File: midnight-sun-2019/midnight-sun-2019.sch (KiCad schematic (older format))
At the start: 71 parts, among them J1 Conn_02x02_Odd_Even, J2 USB_B_Micro, SW1 SW_SPDT, SW2 SW_SPDT, SW3 SW_SPDT, U1 74HC14, U10 74HC14, U11 74HC86, U12 74HC86, U13 74HC86, U14 74HC86, U15 74HC14, U16 74HC14, U2 74HC595, U3 74HC595, U4 74HC595, U5 74HC86, U6 74HC86, U7 74HC86, U8 74HC86, U9 74HC14

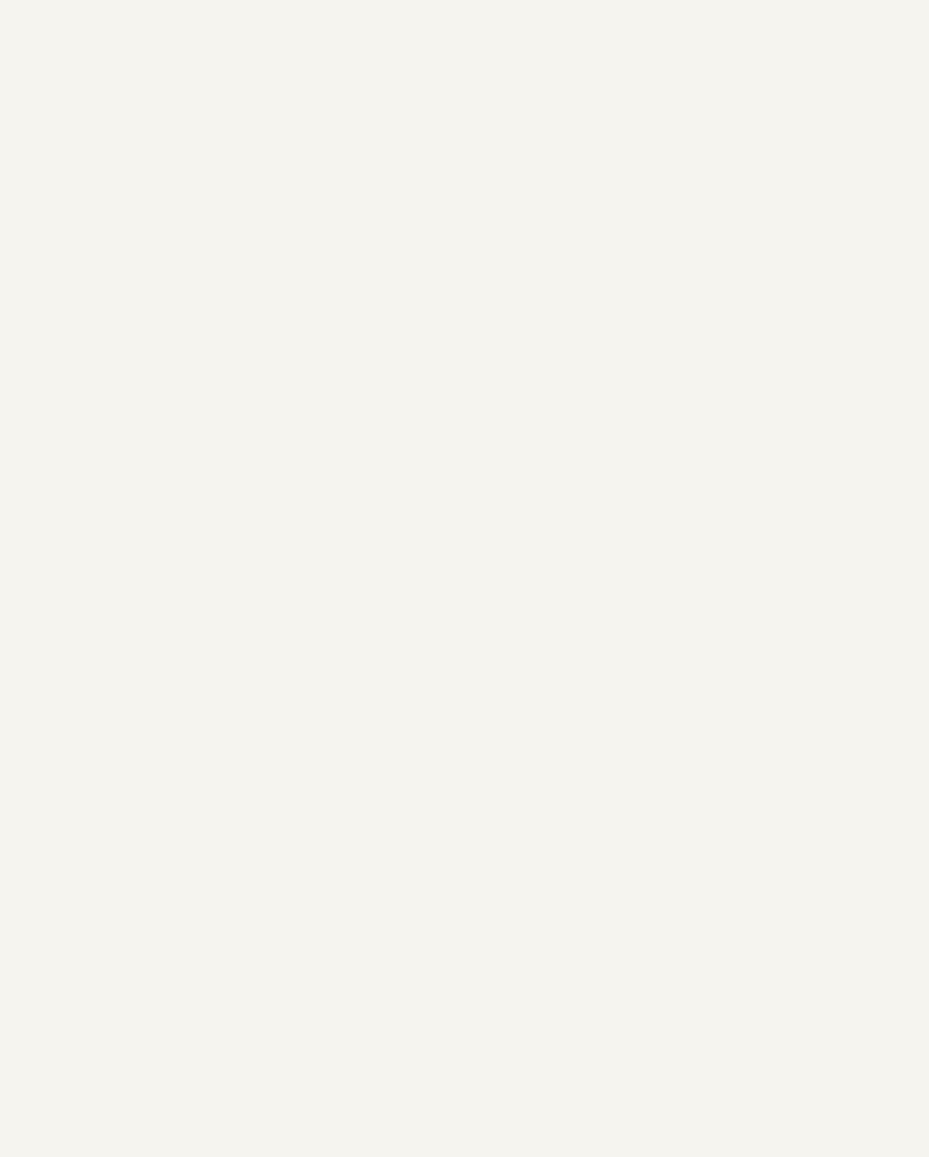
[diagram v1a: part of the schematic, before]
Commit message: Add GND and VCC connections to ICs...
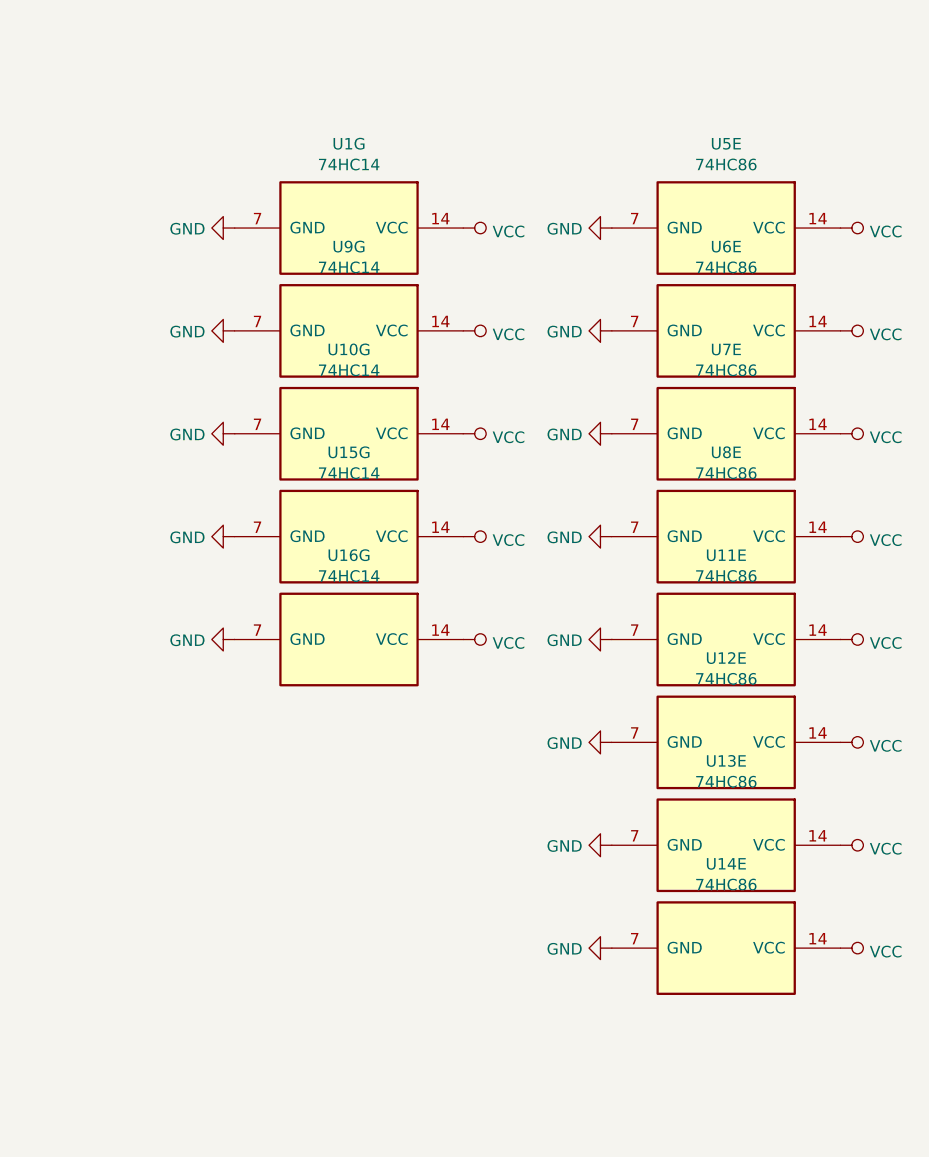
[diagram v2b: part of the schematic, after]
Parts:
- added unit 7 of U1
- added unit 7 of U10
- added unit 5 of U11
- added unit 5 of U12
- added unit 5 of U13
- added unit 5 of U14
- added unit 7 of U15
- added unit 7 of U16
- added unit 5 of U5
- added unit 5 of U6
- added unit 5 of U7
- added unit 5 of U8
- added unit 7 of U9
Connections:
- net GND: now also U1.7 (GND), U10.7 (GND), U11.7 (GND), U12.7 (GND), U13.7 (GND), U14.7 (GND), U15.7 (GND), U16.7 (GND), U5.7 (GND), U6.7 (GND), U7.7 (GND), U8.7 (GND), U9.7 (GND)
- net VCC: now also U1.14 (VCC), U10.14 (VCC), U11.14 (VCC), U12.14 (VCC), U13.14 (VCC), U14.14 (VCC), U15.14 (VCC), U16.14 (VCC), U5.14 (VCC), U6.14 (VCC), U7.14 (VCC), U8.14 (VCC), U9.14 (VCC)

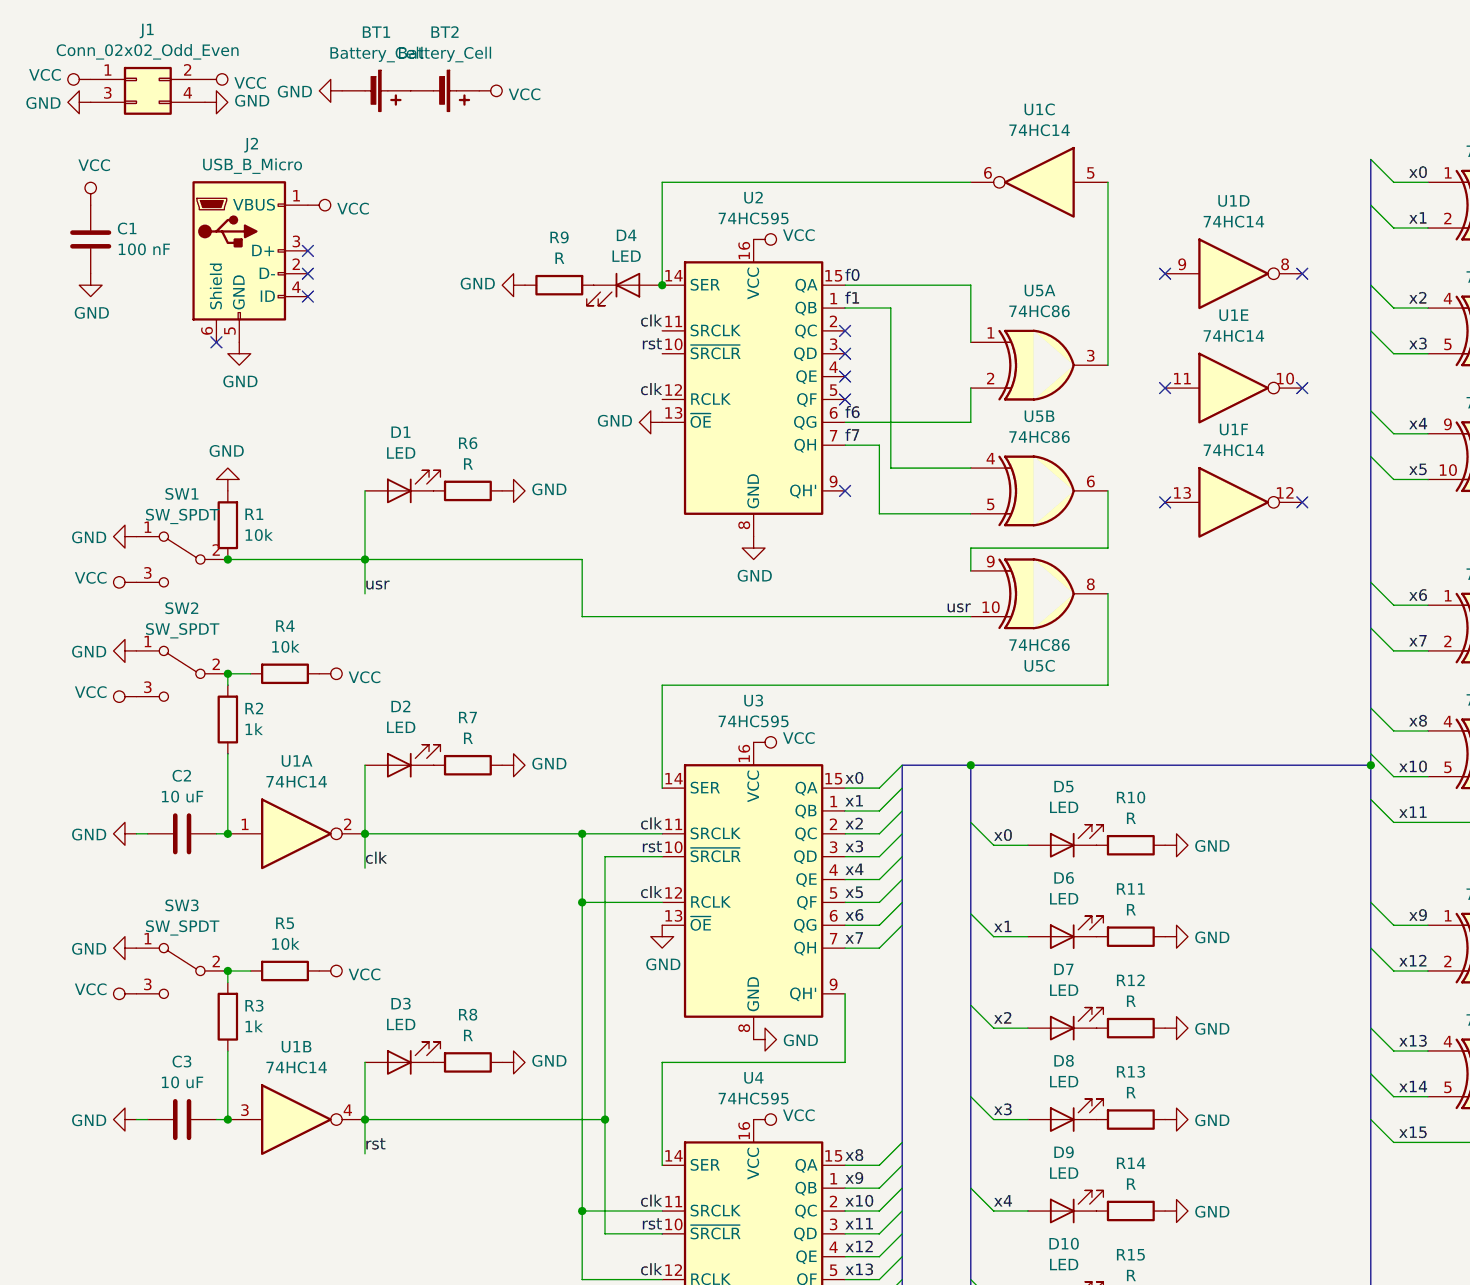
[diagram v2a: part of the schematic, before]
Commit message: Add debounce to SW1
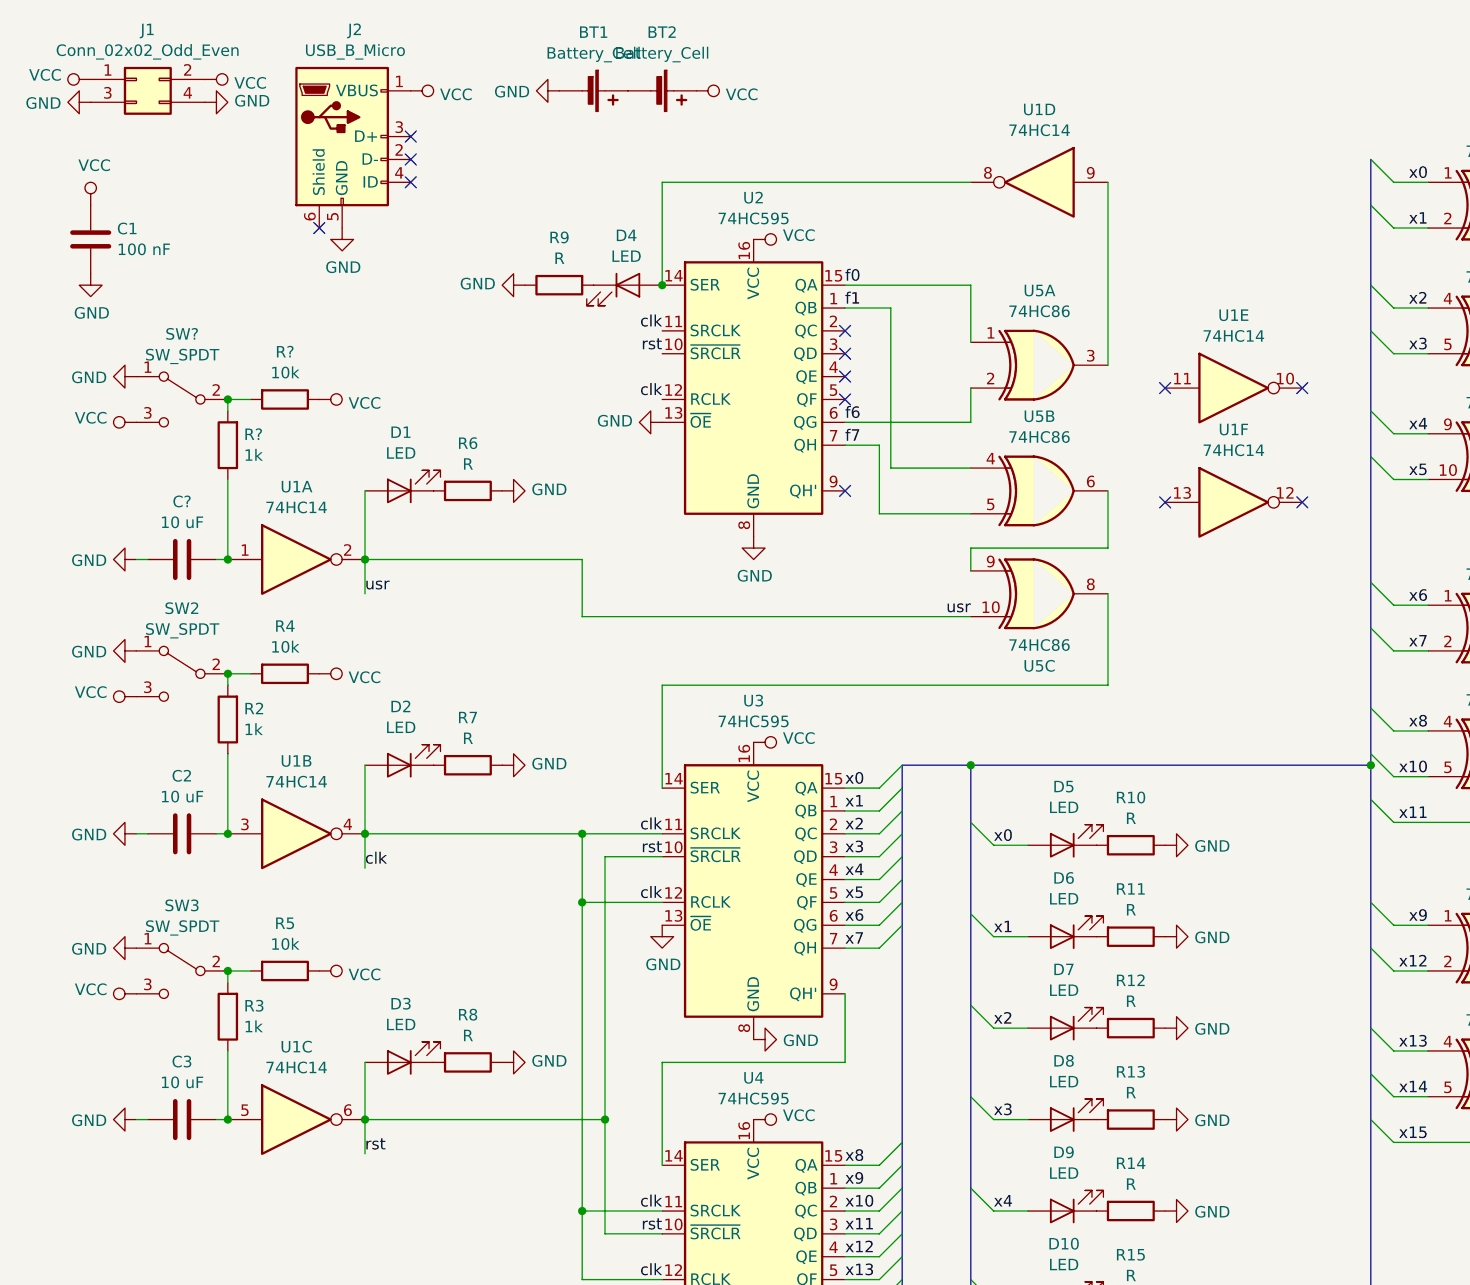
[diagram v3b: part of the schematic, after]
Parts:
- removed R1: 10k, Resistor_THT:R_Axial_DIN0207_L6.3mm_D2.5mm_P7.62mm_Horizontal, symbol Device:R
- removed SW1: SW_SPDT, electrokit:SW_SPDT_MTS-102-A2, symbol Switch:SW_SPDT
- added C?: 10 uF, Capacitor_THT:CP_Radial_D5.0mm_P2.00mm, symbol Device:C
- added R?: 10k, Resistor_THT:R_Axial_DIN0207_L6.3mm_D2.5mm_P7.62mm_Horizontal, symbol Device:R
- added R?: 1k, Resistor_THT:R_Axial_DIN0207_L6.3mm_D2.5mm_P7.62mm_Horizontal, symbol Device:R
- added SW?: SW_SPDT, electrokit:SW_PUSH_DPDT_CW_Industries_GPBS850L, symbol Switch:SW_SPDT
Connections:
- net GND: now also C?.2, SW?.1 (A)
- net VCC: now also R?.1, SW?.3 (C)
- net clk: now also U1.4; no longer U1.2
- net rst: now also U1.6; no longer U1.4
- net usr: now also U1.2
- net at U5.3: now also U1.9; no longer U1.5
- net at D4.2 (A), U2.14 (SER): now also U1.8; no longer U1.6
- net at C2.1, R2.1: now also U1.3; no longer U1.1
- net at C3.1, R3.1: now also U1.5; no longer U1.3
- new net: R?.2, R?.2, SW?.2 (B)
- new net: C?.1, R?.1, U1.1
- no-connect marks 26 -> 24
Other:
- moved on the sheet: BT1, BT2, J2, U1A, U1B, U1C, U1D
